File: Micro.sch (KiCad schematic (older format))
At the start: 0 parts

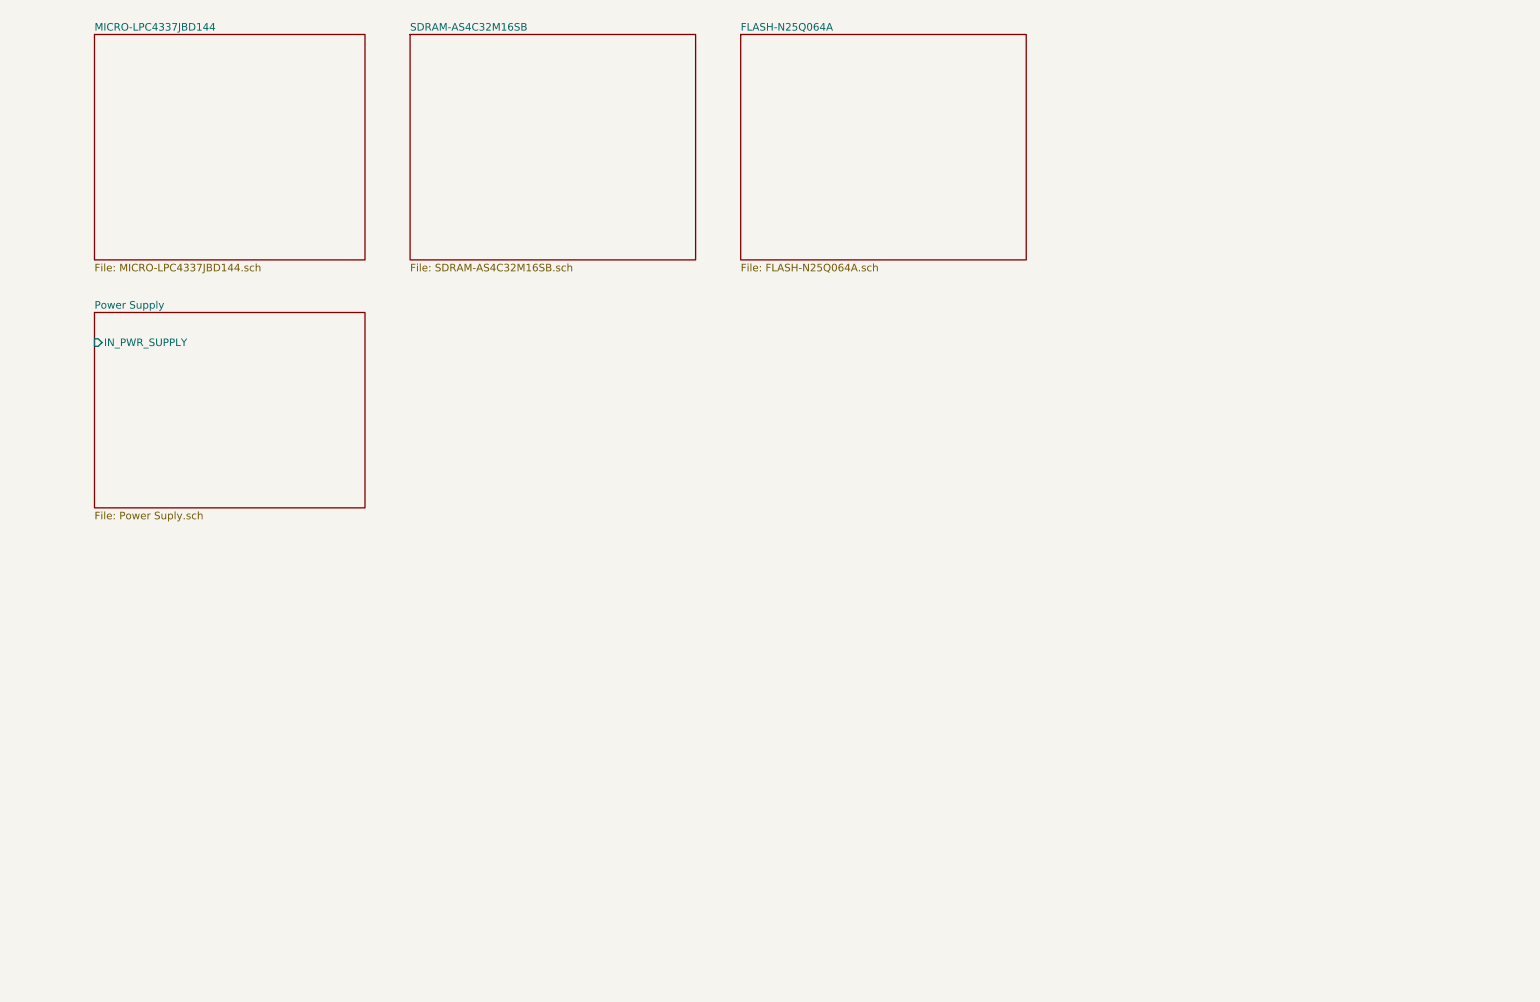
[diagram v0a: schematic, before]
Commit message: LPC + RAM + ROM Progress
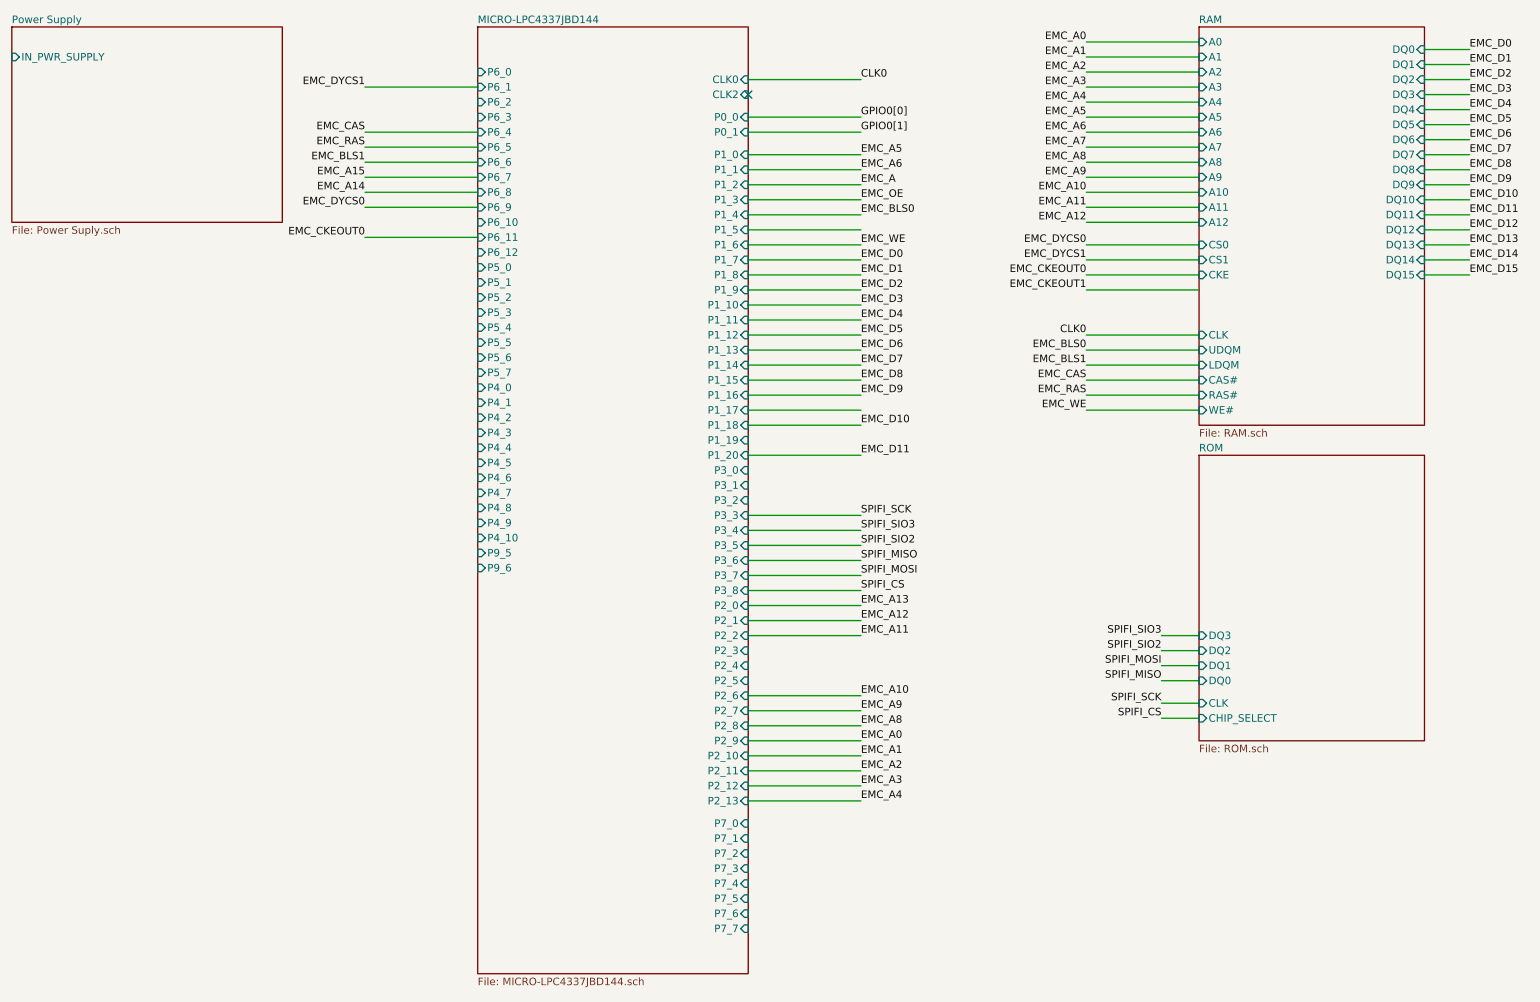
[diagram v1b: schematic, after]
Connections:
- no-connect marks 0 -> 1
